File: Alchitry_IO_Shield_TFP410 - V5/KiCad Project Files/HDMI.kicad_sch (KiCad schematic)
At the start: 19 parts, among them J1 HDMI_A_1.4, U2 TFP410

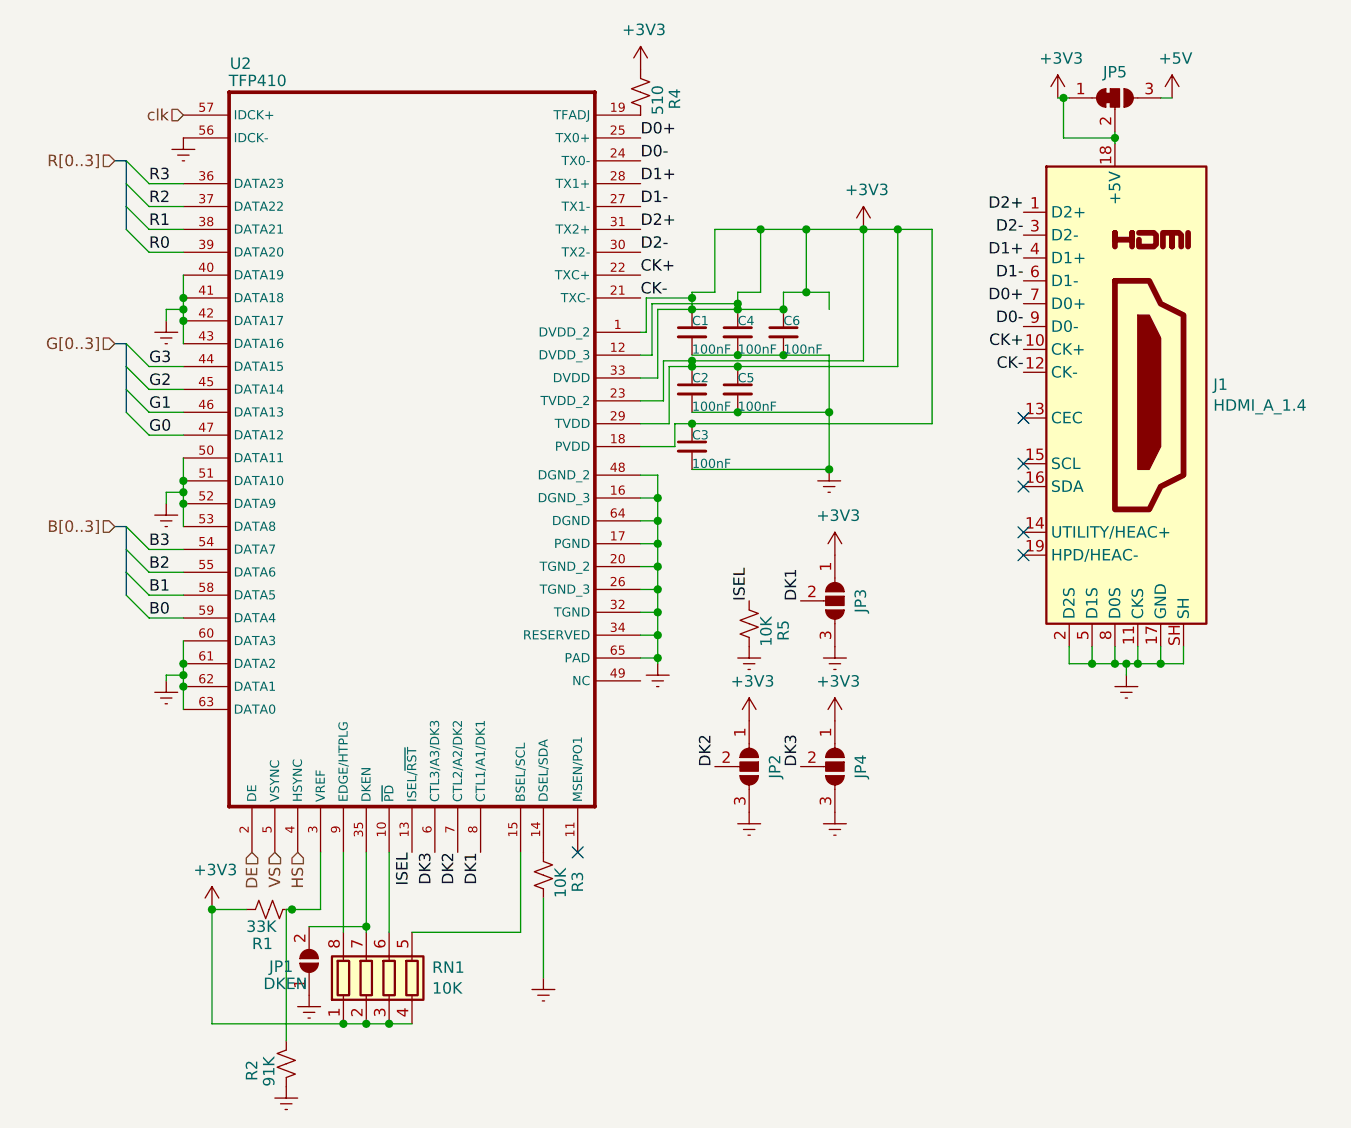
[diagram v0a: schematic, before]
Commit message: started new shield
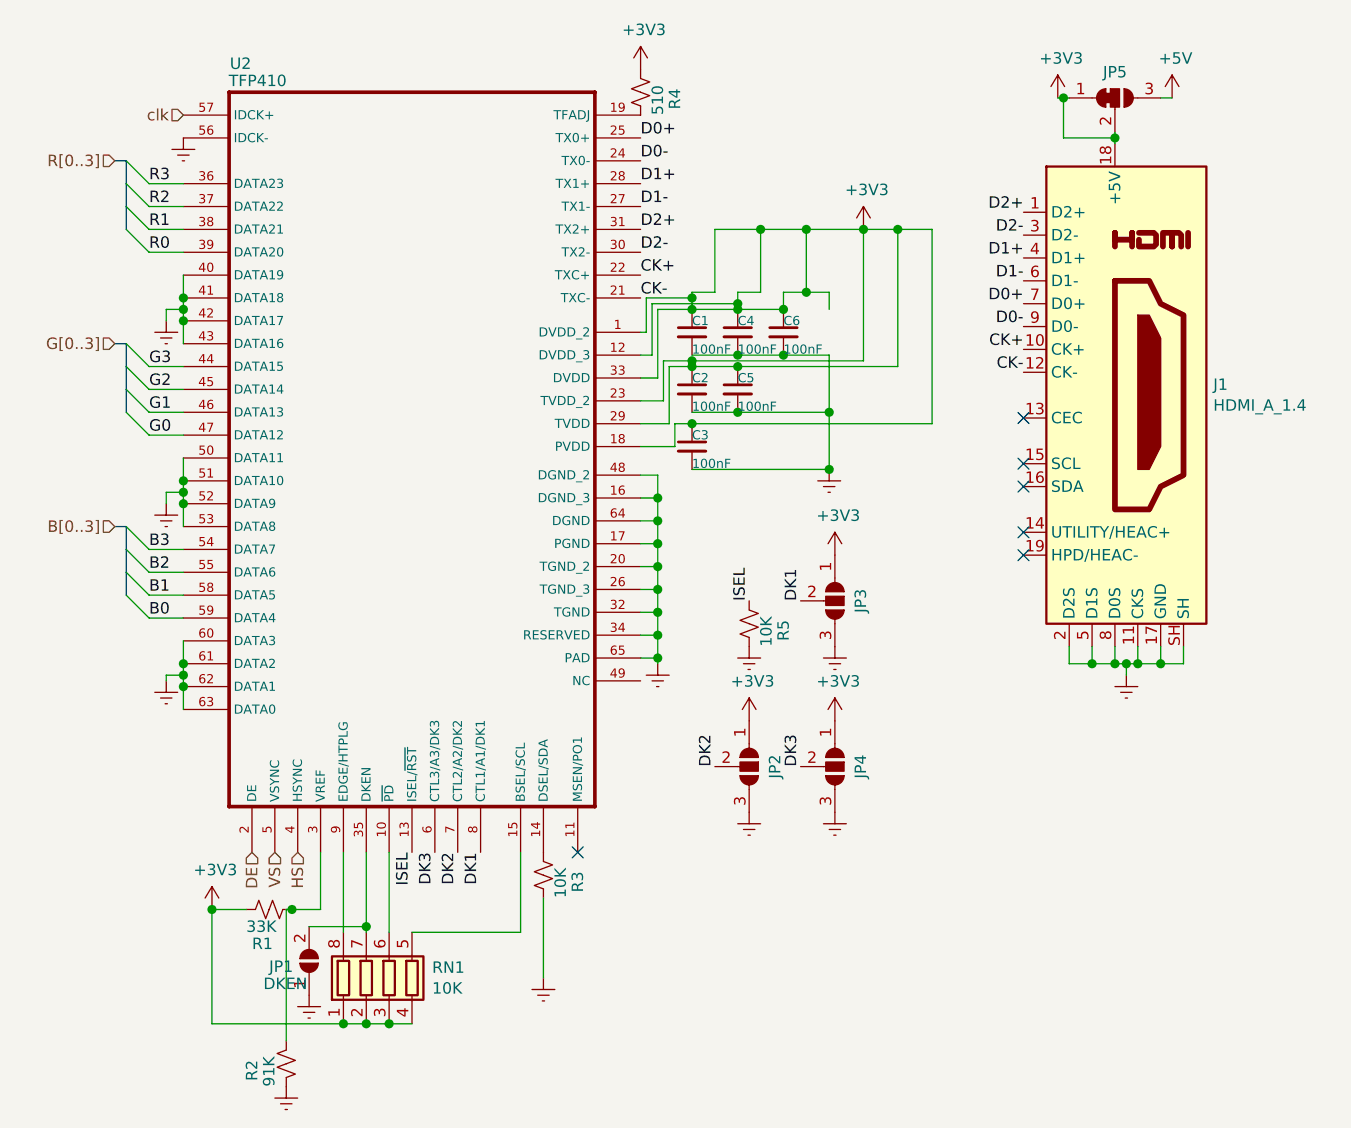
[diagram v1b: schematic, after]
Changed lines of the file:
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@@
-(kicad_sch (version 20200714) (host eeschema "(5.99.0-2416-g010316457)")
-  (page 1 3)
+(kicad_sch (version 20200714) (host eeschema "(5.99.0-2671-gfc0a358ba)")
+  (page 2 3)
   (paper "A4")
-  (junction (at 95.25 67.945) (diameter 0) (color 0 0 0 0))
-  (junction (at 95.25 69.215) (diameter 0) (color 0 0 0 0))
-  (junction (at 95.25 70.485) (diameter 0) (color 0 0 0 0))
-  (junction (at 95.25 88.265) (diameter 0) (color 0 0 0 0))
-  (junction (at 95.25 89.535) (diameter 0) (color 0 0 0 0))
-  (junction (at 95.25 90.805) (diameter 0) (color 0 0 0 0))
-  (junction (at 95.25 108.585) (diameter 0) (color 0 0 0 0))
-  (junction (at 95.25 109.855) (diameter 0) (color 0 0 0 0))
-  (junction (at 95.25 111.125) (diameter 0) (color 0 0 0 0))
-  (junction (at 98.425 135.89) (diameter 0) (color 0 0 0 0))
-  (junction (at 107.315 135.89) (diameter 0) (color 0 0 0 0))
-  (junction (at 113.03 148.59) (diameter 0) (color 0 0 0 0))
-  (junction (at 115.57 137.795) (diameter 0) (color 0 0 0 0))
-  (junction (at 115.57 148.59) (diameter 0) (color 0 0 0 0))
-  (junction (at 118.11 148.59) (diameter 0) (color 0 0 0 0))
-  (junction (at 147.955 90.17) (diameter 0) (color 0 0 0 0))
-  (junction (at 147.955 92.71) (diameter 0) (color 0 0 0 0))
-  (junction (at 147.955 95.25) (diameter 0) (color 0 0 0 0))
-  (junction (at 147.955 97.79) (diameter 0) (color 0 0 0 0))
-  (junction (at 147.955 100.33) (diameter 0) (color 0 0 0 0))
-  (junction (at 147.955 102.87) (diameter 0) (color 0 0 0 0))
-  (junction (at 147.955 105.41) (diameter 0) (color 0 0 0 0))
-  (junction (at 147.955 107.95) (diameter 0) (color 0 0 0 0))
-  (junction (at 151.765 67.945) (diameter 0) (color 0 0 0 0))
-  (junction (at 151.765 69.215) (diameter 0) (color 0 0 0 0))
-  (junction (at 151.765 74.93) (diameter 0) (color 0 0 0 0))
-  (junction (at 151.765 75.565) (diameter 0) (color 0 0 0 0))
-  (junction (at 151.765 81.915) (diameter 0) (color 0 0 0 0))
-  (junction (at 156.845 68.58) (diameter 0) (color 0 0 0 0))
-  (junction (at 156.845 69.215) (diameter 0) (color 0 0 0 0))
-  (junction (at 156.845 74.295) (diameter 0) (color 0 0 0 0))
-  (junction (at 156.845 75.565) (diameter 0) (color 0 0 0 0))
-  (junction (at 156.845 80.645) (diameter 0) (color 0 0 0 0))
-  (junction (at 159.385 60.325) (diameter 0) (color 0 0 0 0))
-  (junction (at 161.925 69.215) (diameter 0) (color 0 0 0 0))
-  (junction (at 161.925 74.295) (diameter 0) (color 0 0 0 0))
-  (junction (at 164.465 60.325) (diameter 0) (color 0 0 0 0))
-  (junction (at 164.465 67.31) (diameter 0) (color 0 0 0 0))
-  (junction (at 167.005 80.645) (diameter 0) (color 0 0 0 0))
-  (junction (at 167.005 86.995) (diameter 0) (color 0 0 0 0))
-  (junction (at 170.815 60.325) (diameter 0) (color 0 0 0 0))
-  (junction (at 174.625 60.325) (diameter 0) (color 0 0 0 0))
-  (junction (at 193.04 45.72) (diameter 0) (color 0 0 0 0))
-  (junction (at 196.215 108.585) (diameter 0) (color 0 0 0 0))
-  (junction (at 198.755 50.165) (diameter 0) (color 0 0 0 0))
-  (junction (at 198.755 108.585) (diameter 0) (color 0 0 0 0))
-  (junction (at 200.025 108.585) (diameter 0) (color 0 0 0 0))
-  (junction (at 201.295 108.585) (diameter 0) (color 0 0 0 0))
-  (junction (at 203.835 108.585) (diameter 0) (color 0 0 0 0))
-  (no_connect (at 188.595 86.36))
-  (no_connect (at 188.595 88.9))
-  (no_connect (at 188.595 93.98))
-  (no_connect (at 188.595 96.52))
+  (junction (at 95.25 67.945) (diameter 1.016) (color 0 0 0 0))
+  (junction (at 95.25 69.215) (diameter 1.016) (color 0 0 0 0))
+  (junction (at 95.25 70.485) (diameter 1.016) (color 0 0 0 0))
+  (junction (at 95.25 88.265) (diameter 1.016) (color 0 0 0 0))
+  (junction (at 95.25 89.535) (diameter 1.016) (color 0 0 0 0))
+  (junction (at 95.25 90.805) (diameter 1.016) (color 0 0 0 0))
+  (junction (at 95.25 108.585) (diameter 1.016) (color 0 0 0 0))
+  (junction (at 95.25 109.855) (diameter 1.016) (color 0 0 0 0))
+  (junction (at 95.25 111.125) (diameter 1.016) (color 0 0 0 0))
+  (junction (at 98.425 135.89) (diameter 1.016) (color 0 0 0 0))
+  (junction (at 107.315 135.89) (diameter 1.016) (color 0 0 0 0))
+  (junction (at 113.03 148.59) (diameter 1.016) (color 0 0 0 0))
+  (junction (at 115.57 137.795) (diameter 1.016) (color 0 0 0 0))
+  (junction (at 115.57 148.59) (diameter 1.016) (color 0 0 0 0))
+  (junction (at 118.11 148.59) (diameter 1.016) (color 0 0 0 0))
+  (junction (at 147.955 90.17) (diameter 1.016) (color 0 0 0 0))
+  (junction (at 147.955 92.71) (diameter 1.016) (color 0 0 0 0))
+  (junction (at 147.955 95.25) (diameter 1.016) (color 0 0 0 0))
+  (junction (at 147.955 97.79) (diameter 1.016) (color 0 0 0 0))
+  (junction (at 147.955 100.33) (diameter 1.016) (color 0 0 0 0))
+  (junction (at 147.955 102.87) (diameter 1.016) (color 0 0 0 0))
+  (junction (at 147.955 105.41) (diameter 1.016) (color 0 0 0 0))
+  (junction (at 147.955 107.95) (diameter 1.016) (color 0 0 0 0))
+  (junction (at 151.765 67.945) (diameter 1.016) (color 0 0 0 0))
+  (junction (at 151.765 69.215) (diameter 1.016) (color 0 0 0 0))
+  (junction (at 151.765 74.93) (diameter 1.016) (color 0 0 0 0))
+  (junction (at 151.765 75.565) (diameter 1.016) (color 0 0 0 0))
+  (junction (at 151.765 81.915) (diameter 1.016) (color 0 0 0 0))
+  (junction (at 156.845 68.58) (diameter 1.016) (color 0 0 0 0))
+  (junction (at 156.845 69.215) (diameter 1.016) (color 0 0 0 0))
+  (junction (at 156.845 74.295) (diameter 1.016) (color 0 0 0 0))
+  (junction (at 156.845 75.565) (diameter 1.016) (color 0 0 0 0))
+  (junction (at 156.845 80.645) (diameter 1.016) (color 0 0 0 0))
+  (junction (at 159.385 60.325) (diameter 1.016) (color 0 0 0 0))
+  (junction (at 161.925 69.215) (diameter 1.016) (color 0 0 0 0))
+  (junction (at 161.925 74.295) (diameter 1.016) (color 0 0 0 0))
+  (junction (at 164.465 60.325) (diameter 1.016) (color 0 0 0 0))
+  (junction (at 164.465 67.31) (diameter 1.016) (color 0 0 0 0))
+  (junction (at 167.005 80.645) (diameter 1.016) (color 0 0 0 0))
+  (junction (at 167.005 86.995) (diameter 1.016) (color 0 0 0 0))
+  (junction (at 170.815 60.325) (diameter 1.016) (color 0 0 0 0))
+  (junction (at 174.625 60.325) (diameter 1.016) (color 0 0 0 0))
+  (junction (at 193.04 45.72) (diameter 1.016) (color 0 0 0 0))
+  (junction (at 196.215 108.585) (diameter 1.016) (color 0 0 0 0))
+  (junction (at 198.755 50.165) (diameter 1.016) (color 0 0 0 0))
+  (junction (at 198.755 108.585) (diameter 1.016) (color 0 0 0 0))
+  (junction (at 200.025 108.585) (diameter 1.016) (color 0 0 0 0))
+  (junction (at 201.295 108.585) (diameter 1.016) (color 0 0 0 0))
+  (junction (at 203.835 108.585) (diameter 1.016) (color 0 0 0 0))
   (no_connect (at 139.065 129.54))
   (no_connect (at 188.595 81.28))
+  (no_connect (at 188.595 88.9))
+  (no_connect (at 188.595 96.52))
+  (no_connect (at 188.595 93.98))
+  (no_connect (at 188.595 86.36))
   (bus_entry (at 88.9 52.705) (size 2.54 2.54)
     (stroke (width 0.1524) (type solid) (color 0 0 0 0))
@@
     (stroke (width 0) (type solid) (color 0 0 0 0))
   )
-  (bus (pts (xy 88.9 52.705) (xy 88.9 57.785))
+  (bus (pts (xy 88.9 52.705) (xy 88.9 55.245))
+    (stroke (width 0) (type solid) (color 0 0 0 0))
+  )
+  (bus (pts (xy 88.9 55.245) (xy 88.9 57.785))
     (stroke (width 0) (type solid) (color 0 0 0 0))
   )
@@
     (stroke (width 0) (type solid) (color 0 0 0 0))
   )
-  (bus (pts (xy 88.9 75.565) (xy 88.9 80.645))
+  (bus (pts (xy 88.9 75.565) (xy 88.9 78.105))
+    (stroke (width 0) (type solid) (color 0 0 0 0))
+  )
+  (bus (pts (xy 88.9 78.105) (xy 88.9 80.645))
     (stroke (width 0) (type solid) (color 0 0 0 0))
   )
@@
     (stroke (width 0) (type solid) (color 0 0 0 0))
   )
-  (bus (pts (xy 88.9 93.345) (xy 88.9 98.425))
-    (stroke (width 0) (type solid) (color 0 0 0 0))
-  )
+  (bus (pts (xy 88.9 93.345) (xy 88.9 95.885))
+    (stroke (width 0) (type solid) (color 0 0 0 0))
+  )
+  (bus (pts (xy 88.9 95.885) (xy 88.9 98.425))
+    (stroke (width 0) (type solid) (color 0 0 0 0))
+  )
